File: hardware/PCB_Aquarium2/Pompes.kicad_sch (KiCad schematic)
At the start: 8 parts, among them J21 Conn_01x02, J22 Conn_01x02, J23 Conn_01x02, J24 Conn_01x02, Q1 NPN, Q2 NPN

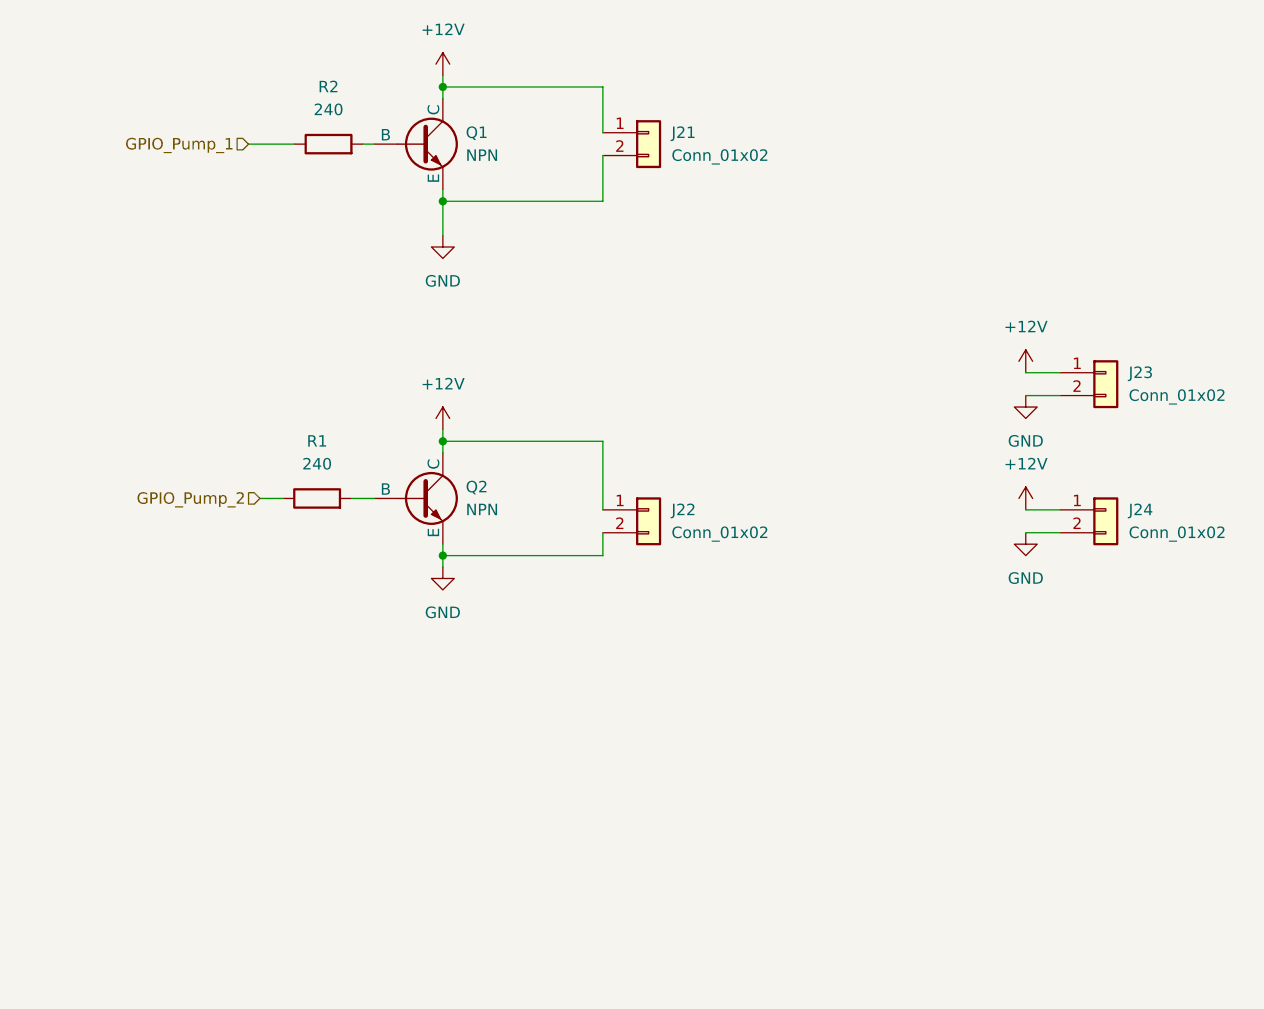
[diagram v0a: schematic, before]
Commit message: PCBs v3
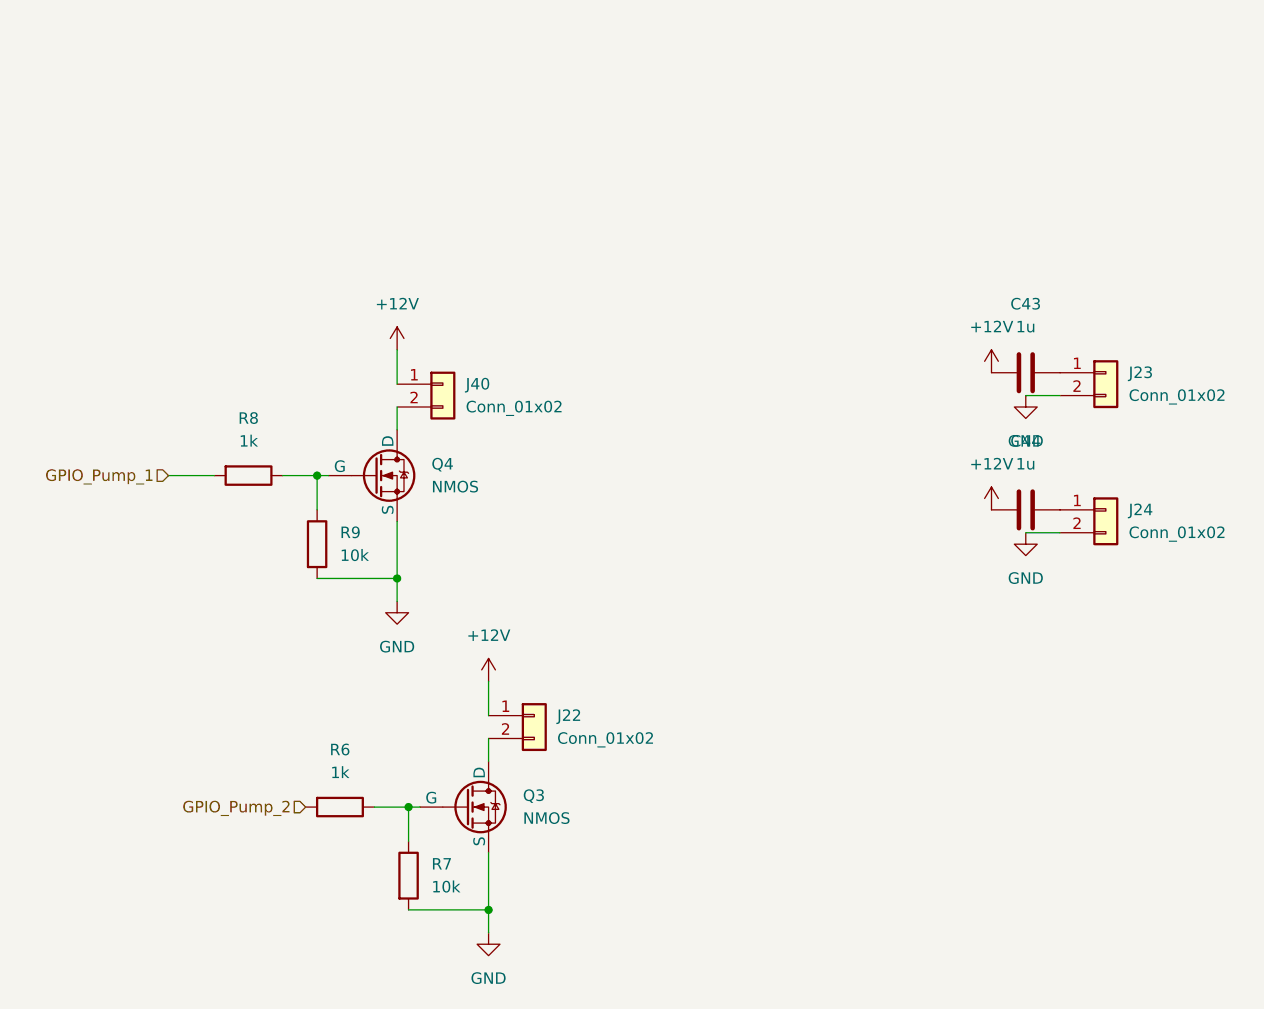
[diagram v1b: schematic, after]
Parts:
- removed J21: Conn_01x02, Connector_JST:JST_EH_B2B-EH-A_1x02_P2.50mm_Vertical, symbol Connector_Generic:Conn_01x02
- removed Q1, Q2: NPN, Package_TO_SOT_SMD:TSOT-23, symbol Simulation_SPICE:NPN
- removed R1, R2: 240, Resistor_SMD:R_0805_2012Metric, symbol Device:R
- added C43, C44: 1u, Capacitor_SMD:C_0603_1608Metric, symbol Device:C
- added J40: Conn_01x02, Connector_JST:JST_EH_B2B-EH-A_1x02_P2.50mm_Vertical, symbol Connector_Generic:Conn_01x02
- added Q3, Q4: NMOS, Package_TO_SOT_SMD:SOT-23, symbol Simulation_SPICE:NMOS
- added R6, R8: 1k, Resistor_SMD:R_0402_1005Metric, symbol Device:R
- added R7, R9: 10k, Resistor_SMD:R_0402_1005Metric, symbol Device:R
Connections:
- net +12V: now also C43.1, C44.1, J40.1 (Pin_1); no longer J23.1 (Pin_1), J24.1 (Pin_1)
- net GND: now also Q3.3 (S), Q4.3 (S), R7.2, R9.2; no longer J22.2 (Pin_2)
- net GPIO_Pump_1: now also R8.2
- net GPIO_Pump_2: now also R6.2
- new net: C43.2, J23.1 (Pin_1)
- new net: J40.2 (Pin_2), Q4.1 (D)
- new net: J22.2 (Pin_2), Q3.1 (D)
- new net: Q3.2 (G), R6.1, R7.1
- new net: Q4.2 (G), R8.1, R9.1
- new net: C44.2, J24.1 (Pin_1)
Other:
- moved on the sheet: J22
